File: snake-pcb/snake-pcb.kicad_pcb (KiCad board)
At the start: 4 copper layers, 38.1 x 57.2 mm, 26 parts, among them J1 USB_C, SW1 SW_Push, U1 STM32F072CBT6, U3 XC6206, U4 USBLC6-2SC6

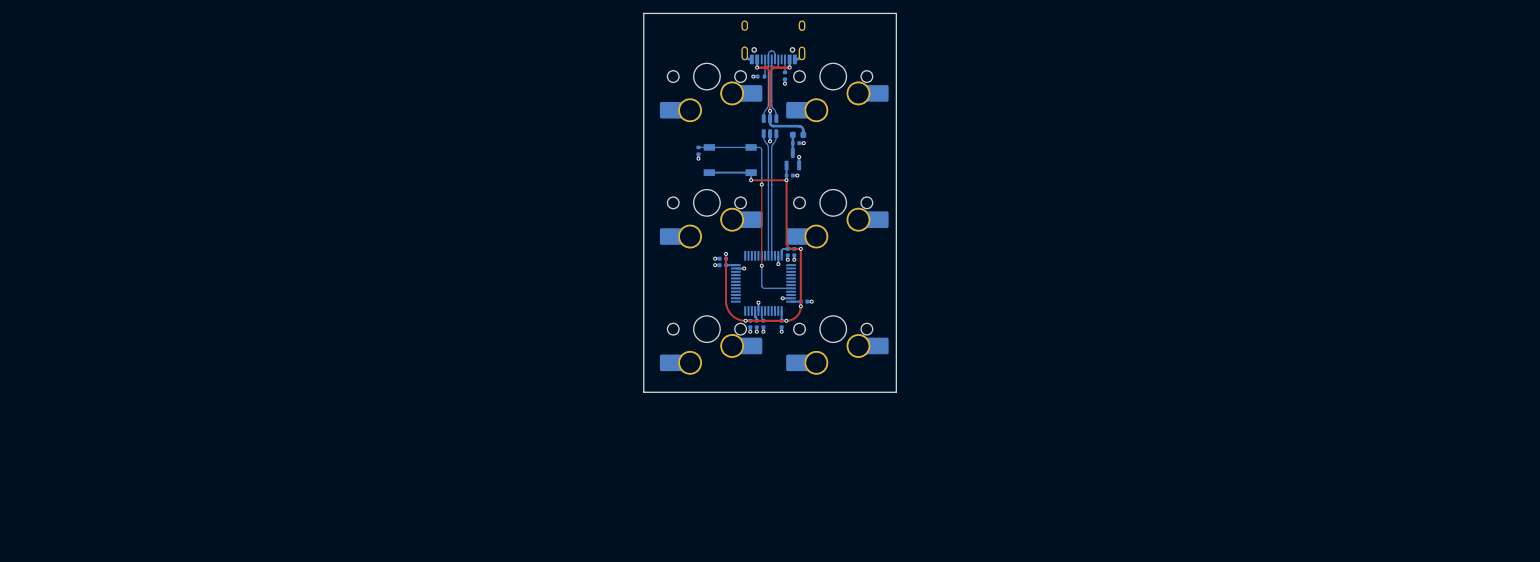
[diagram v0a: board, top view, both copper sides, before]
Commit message: pcb almost finished!
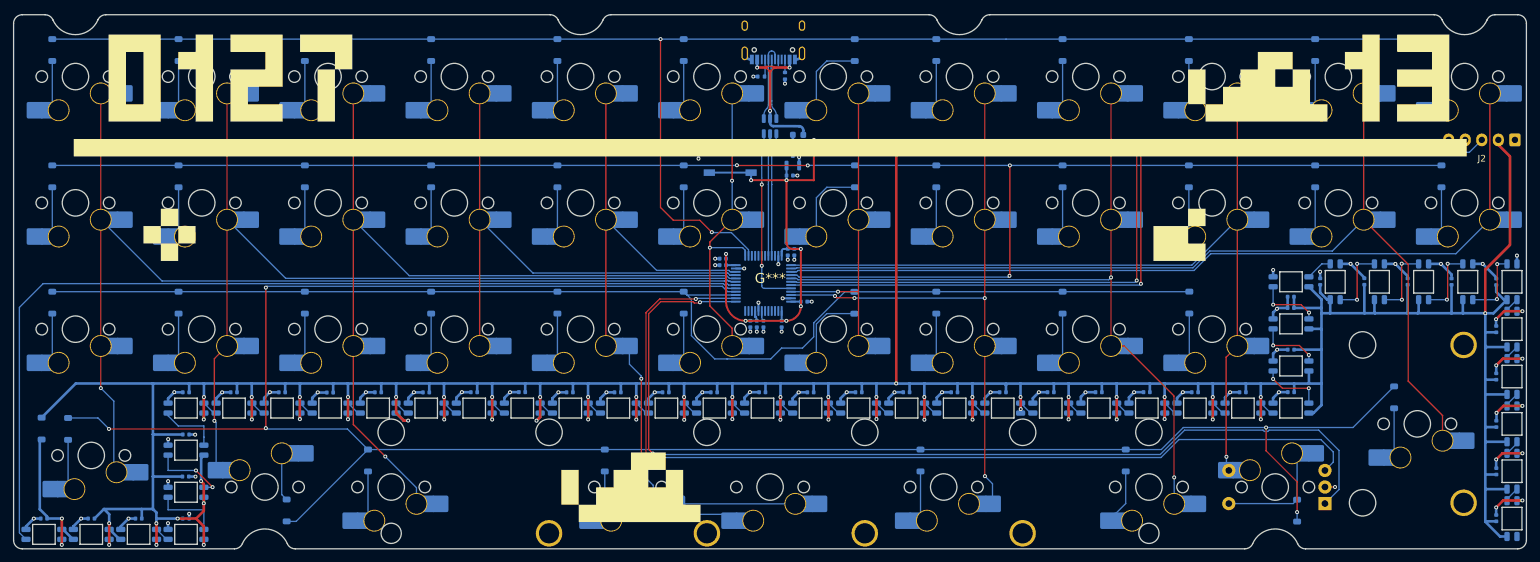
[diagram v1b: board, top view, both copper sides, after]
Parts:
- removed REF** (x6): MX_1.00u_PG151101S11, ScottoKeebs_Scotto:MX_Hotswap_1.00u
- added CapLED1: 100nF, ScottoKeebs_Components:Capacitor_0402, B.Cu at (41.6, 146.6)
- added CapLED10: 100nF, ScottoKeebs_Components:Capacitor_0402, B.Cu at (84.8, 127.6)
- added CapLED11: 100nF, ScottoKeebs_Components:Capacitor_0402, B.Cu at (92.0, 127.6)
- added CapLED12: 100nF, ScottoKeebs_Components:Capacitor_0402, B.Cu at (99.3, 127.6)
- added CapLED13: 100nF, ScottoKeebs_Components:Capacitor_0402, B.Cu at (106.5, 127.6)
- added CapLED14: 100nF, ScottoKeebs_Components:Capacitor_0402, B.Cu at (113.7, 127.5)
- added CapLED15: 100nF, ScottoKeebs_Components:Capacitor_0402, B.Cu at (120.9, 127.6)
- added CapLED16: 100nF, ScottoKeebs_Components:Capacitor_0402, B.Cu at (128.2, 127.6)
- added CapLED17: 100nF, ScottoKeebs_Components:Capacitor_0402, B.Cu at (135.4, 127.6)
- added CapLED18: 100nF, ScottoKeebs_Components:Capacitor_0402, B.Cu at (142.7, 127.6)
- added CapLED19: 100nF, ScottoKeebs_Components:Capacitor_0402, B.Cu at (150.0, 127.6)
- added CapLED2: 100nF, ScottoKeebs_Components:Capacitor_0402, B.Cu at (48.8, 146.6)
- added CapLED20: 100nF, ScottoKeebs_Components:Capacitor_0402, B.Cu at (157.3, 127.6)
- added CapLED21: 100nF, ScottoKeebs_Components:Capacitor_0402, B.Cu at (164.5, 127.6)
- added CapLED22: 100nF, ScottoKeebs_Components:Capacitor_0402, B.Cu at (171.7, 127.6)
- added CapLED23: 100nF, ScottoKeebs_Components:Capacitor_0402, B.Cu at (179.0, 127.6)
- added CapLED24: 100nF, ScottoKeebs_Components:Capacitor_0402, B.Cu at (186.3, 127.6)
- added CapLED25: 100nF, ScottoKeebs_Components:Capacitor_0402, B.Cu at (193.5, 127.6)
- added CapLED26: 100nF, ScottoKeebs_Components:Capacitor_0402, B.Cu at (200.7, 127.6)
- added CapLED27: 100nF, ScottoKeebs_Components:Capacitor_0402, B.Cu at (208.0, 127.6)
- added CapLED28: 100nF, ScottoKeebs_Components:Capacitor_0402, B.Cu at (215.3, 127.6)
- added CapLED29: 100nF, ScottoKeebs_Components:Capacitor_0402, B.Cu at (222.5, 127.6)
- added CapLED3: 100nF, ScottoKeebs_Components:Capacitor_0402, B.Cu at (55.9, 146.6)
- added CapLED30: 100nF, ScottoKeebs_Components:Capacitor_0402, B.Cu at (229.7, 127.6)
- added CapLED31: 100nF, ScottoKeebs_Components:Capacitor_0402, B.Cu at (229.7, 121.1)
- added CapLED32: 100nF, ScottoKeebs_Components:Capacitor_0402, B.Cu at (229.7, 114.9)
- added CapLED33: 100nF, ScottoKeebs_Components:Capacitor_0402, B.Cu at (229.7, 113.2)
- added CapLED34: 100nF, ScottoKeebs_Components:Capacitor_0402, B.Cu at (234.1, 110.9)
- added CapLED35: 100nF, ScottoKeebs_Components:Capacitor_0402, B.Cu at (240.8, 110.9)
- added CapLED36: 100nF, ScottoKeebs_Components:Capacitor_0402, B.Cu at (247.3, 110.9)
- added CapLED37: 100nF, ScottoKeebs_Components:Capacitor_0402, B.Cu at (254.0, 110.9)
- added CapLED38: 100nF, ScottoKeebs_Components:Capacitor_0402, B.Cu at (260.7, 110.9)
- added CapLED39: 100nF, ScottoKeebs_Components:Capacitor_0402, B.Cu at (260.7, 118.1)
- added CapLED4: 100nF, ScottoKeebs_Components:Capacitor_0402, B.Cu at (63.1, 146.6)
- added CapLED40: 100nF, ScottoKeebs_Components:Capacitor_0402, B.Cu at (260.7, 125.2)
- added CapLED41: 100nF, ScottoKeebs_Components:Capacitor_0402, B.Cu at (260.7, 132.3)
- added CapLED42: 100nF, ScottoKeebs_Components:Capacitor_0402, B.Cu at (260.7, 139.5)
- added CapLED43: 100nF, ScottoKeebs_Components:Capacitor_0402, B.Cu at (260.7, 146.6)
- added CapLED5: 100nF, ScottoKeebs_Components:Capacitor_0402, B.Cu at (63.0, 140.3)
- added CapLED6: 100nF, ScottoKeebs_Components:Capacitor_0402, B.Cu at (63.1, 133.9)
- added CapLED7: 100nF, ScottoKeebs_Components:Capacitor_0402, B.Cu at (63.1, 127.6)
- added CapLED8: 100nF, ScottoKeebs_Components:Capacitor_0402, B.Cu at (70.3, 127.6)
- added CapLED9: 100nF, ScottoKeebs_Components:Capacitor_0402, B.Cu at (77.5, 127.6)
- added D1: 1N4148W, Diode_SMD:D_SOD-123, B.Cu at (42.9, 76.0)
- added D10: 1N4148W, Diode_SMD:D_SOD-123, B.Cu at (214.3, 76.0)
- added D11: 1N4148W, Diode_SMD:D_SOD-123, B.Cu at (233.4, 76.0)
- added D12: 1N4148W, Diode_SMD:D_SOD-123, B.Cu at (252.4, 76.0)
- added D13: 1N4148W, Diode_SMD:D_SOD-123, B.Cu at (42.9, 95.0)
- added D14: 1N4148W, Diode_SMD:D_SOD-123, B.Cu at (61.9, 95.0)
- added D15: 1N4148W, Diode_SMD:D_SOD-123, B.Cu at (81.0, 95.0)
- added D16: 1N4148W, Diode_SMD:D_SOD-123, B.Cu at (100.0, 95.0)
- added D17: 1N4148W, Diode_SMD:D_SOD-123, B.Cu at (119.1, 95.0)
- added D18: 1N4148W, Diode_SMD:D_SOD-123, B.Cu at (138.1, 95.0)
- added D19: 1N4148W, Diode_SMD:D_SOD-123, B.Cu at (164.0, 95.0)
- added D2: 1N4148W, Diode_SMD:D_SOD-123, B.Cu at (61.9, 76.0)
- added D20: 1N4148W, Diode_SMD:D_SOD-123, B.Cu at (176.2, 95.0)
- added D21: 1N4148W, Diode_SMD:D_SOD-123, B.Cu at (195.3, 95.0)
- added D22: 1N4148W, Diode_SMD:D_SOD-123, B.Cu at (214.3, 95.0)
- added D23: 1N4148W, Diode_SMD:D_SOD-123, B.Cu at (233.4, 95.0)
- added D24: 1N4148W, Diode_SMD:D_SOD-123, B.Cu at (252.4, 95.0)
- added D25: 1N4148W, Diode_SMD:D_SOD-123, B.Cu at (42.9, 114.1)
- added D26: 1N4148W, Diode_SMD:D_SOD-123, B.Cu at (61.9, 114.1)
- added D27: 1N4148W, Diode_SMD:D_SOD-123, B.Cu at (81.0, 114.1)
- added D28: 1N4148W, Diode_SMD:D_SOD-123, B.Cu at (100.0, 114.1)
- added D29: 1N4148W, Diode_SMD:D_SOD-123, B.Cu at (119.1, 114.1)
- added D3: 1N4148W, Diode_SMD:D_SOD-123, B.Cu at (81.0, 76.0)
- added D30: 1N4148W, Diode_SMD:D_SOD-123, B.Cu at (138.1, 114.1)
- added D31: 1N4148W, Diode_SMD:D_SOD-123, B.Cu at (163.9, 114.1)
- added D32: 1N4148W, Diode_SMD:D_SOD-123, B.Cu at (176.2, 114.1)
- added D33: 1N4148W, Diode_SMD:D_SOD-123, B.Cu at (195.3, 114.1)
- added D34: 1N4148W, Diode_SMD:D_SOD-123, B.Cu at (214.4, 114.0)
- added D35: 1N4148W, Diode_SMD:D_SOD-123, B.Cu at (245.3, 128.3)
- added D36: 1N4148W, Diode_SMD:D_SOD-123, B.Cu at (45.3, 133.1)
- added D37: 1N4148W, Diode_SMD:D_SOD-123, B.Cu at (78.2, 145.4)
- added D38: 1N4148W, Diode_SMD:D_SOD-123, B.Cu at (90.5, 137.9)
- added D39: 1N4148W, Diode_SMD:D_SOD-123, B.Cu at (126.2, 137.9)
- added D4: 1N4148W, Diode_SMD:D_SOD-123, B.Cu at (100.0, 76.0)
- added D40: 1N4148W, Diode_SMD:D_SOD-123, B.Cu at (173.9, 137.9)
- added D41: 1N4148W, Diode_SMD:D_SOD-123, B.Cu at (204.8, 137.9)
- added D42: 1N4148W, Diode_SMD:D_SOD-123, B.Cu at (230.7, 145.4)
- added D5: 1N4148W, Diode_SMD:D_SOD-123, B.Cu at (119.1, 76.0)
- added D6: 1N4148W, Diode_SMD:D_SOD-123, B.Cu at (138.1, 76.0)
- added D7: 1N4148W, Diode_SMD:D_SOD-123, B.Cu at (163.9, 76.0)
- added D8: 1N4148W, Diode_SMD:D_SOD-123, B.Cu at (176.2, 76.0)
- added D9: 1N4148W, Diode_SMD:D_SOD-123, B.Cu at (195.3, 76.0)
- added DLED1: 1N4148W, Diode_SMD:D_SOD-123, B.Cu at (41.3, 133.0)
- added G***: LOGO, snake:snake, F.Cu at (151.2, 110.4)
- added J2: Conn_01x05_Socket, Connector_JST:JST_EH_B5B-EH-A_1x05_P2.50mm_Vertical, F.Cu at (263.5, 89.5)
- added LED1: SK6812MINI, ScottoKeebs_Components:LED_SK6812MINI, B.Cu at (41.6, 149.0)
- added LED10: SK6812MINI, ScottoKeebs_Components:LED_SK6812MINI, B.Cu at (84.8, 130.0)
- added LED11: SK6812MINI, ScottoKeebs_Components:LED_SK6812MINI, B.Cu at (92.0, 130.0)
- added LED12: SK6812MINI, ScottoKeebs_Components:LED_SK6812MINI, B.Cu at (99.3, 130.0)
- added LED13: SK6812MINI, ScottoKeebs_Components:LED_SK6812MINI, B.Cu at (106.5, 130.0)
- added LED14: SK6812MINI, ScottoKeebs_Components:LED_SK6812MINI, B.Cu at (113.8, 130.0)
- added LED15: SK6812MINI, ScottoKeebs_Components:LED_SK6812MINI, B.Cu at (121.0, 130.0)
- added LED16: SK6812MINI, ScottoKeebs_Components:LED_SK6812MINI, B.Cu at (128.3, 130.0)
- added LED17: SK6812MINI, ScottoKeebs_Components:LED_SK6812MINI, B.Cu at (135.5, 130.0)
- added LED18: SK6812MINI, ScottoKeebs_Components:LED_SK6812MINI, B.Cu at (142.8, 130.0)
- added LED19: SK6812MINI, ScottoKeebs_Components:LED_SK6812MINI, B.Cu at (150.0, 130.0)
- added LED2: SK6812MINI, ScottoKeebs_Components:LED_SK6812MINI, B.Cu at (48.8, 149.0)
- added LED20: SK6812MINI, ScottoKeebs_Components:LED_SK6812MINI, B.Cu at (157.3, 130.0)
- added LED21: SK6812MINI, ScottoKeebs_Components:LED_SK6812MINI, B.Cu at (164.5, 130.0)
- added LED22: SK6812MINI, ScottoKeebs_Components:LED_SK6812MINI, B.Cu at (171.8, 130.0)
- added LED23: SK6812MINI, ScottoKeebs_Components:LED_SK6812MINI, B.Cu at (179.0, 130.0)
- added LED24: SK6812MINI, ScottoKeebs_Components:LED_SK6812MINI, B.Cu at (186.3, 130.0)
- added LED25: SK6812MINI, ScottoKeebs_Components:LED_SK6812MINI, B.Cu at (193.5, 130.0)
- added LED26: SK6812MINI, ScottoKeebs_Components:LED_SK6812MINI, B.Cu at (200.7, 130.0)
- added LED27: SK6812MINI, ScottoKeebs_Components:LED_SK6812MINI, B.Cu at (208.0, 130.0)
- added LED28: SK6812MINI, ScottoKeebs_Components:LED_SK6812MINI, B.Cu at (215.2, 130.0)
- added LED29: SK6812MINI, ScottoKeebs_Components:LED_SK6812MINI, B.Cu at (222.5, 130.0)
- added LED3: SK6812MINI, ScottoKeebs_Components:LED_SK6812MINI, B.Cu at (55.9, 149.0)
- added LED30: SK6812MINI, ScottoKeebs_Components:LED_SK6812MINI, B.Cu at (229.7, 130.0)
- added LED31: SK6812MINI, ScottoKeebs_Components:LED_SK6812MINI, B.Cu at (229.7, 123.6)
- added LED32: SK6812MINI, ScottoKeebs_Components:LED_SK6812MINI, B.Cu at (229.7, 117.3)
- added LED33: SK6812MINI, ScottoKeebs_Components:LED_SK6812MINI, B.Cu at (229.7, 110.9)
- added LED34: SK6812MINI, ScottoKeebs_Components:LED_SK6812MINI, B.Cu at (236.4, 110.9)
- added LED35: SK6812MINI, ScottoKeebs_Components:LED_SK6812MINI, B.Cu at (243.1, 110.9)
- added LED36: SK6812MINI, ScottoKeebs_Components:LED_SK6812MINI, B.Cu at (249.7, 110.9)
- added LED37: SK6812MINI, ScottoKeebs_Components:LED_SK6812MINI, B.Cu at (256.4, 110.9)
- added LED38: SK6812MINI, ScottoKeebs_Components:LED_SK6812MINI, B.Cu at (263.1, 110.9)
- added LED39: SK6812MINI, ScottoKeebs_Components:LED_SK6812MINI, B.Cu at (263.1, 118.1)
- added LED4: SK6812MINI, ScottoKeebs_Components:LED_SK6812MINI, B.Cu at (63.1, 149.0)
- added LED40: SK6812MINI, ScottoKeebs_Components:LED_SK6812MINI, B.Cu at (263.1, 125.2)
- added LED41: SK6812MINI, ScottoKeebs_Components:LED_SK6812MINI, B.Cu at (263.1, 132.3)
- added LED42: SK6812MINI, ScottoKeebs_Components:LED_SK6812MINI, B.Cu at (263.1, 139.5)
- added LED43: SK6812MINI, ScottoKeebs_Components:LED_SK6812MINI, B.Cu at (263.1, 146.6)
- added LED5: SK6812MINI, ScottoKeebs_Components:LED_SK6812MINI, B.Cu at (63.1, 142.7)
- added LED6: SK6812MINI, ScottoKeebs_Components:LED_SK6812MINI, B.Cu at (63.1, 136.3)
- added LED7: SK6812MINI, ScottoKeebs_Components:LED_SK6812MINI, B.Cu at (63.1, 130.0)
- added LED8: SK6812MINI, ScottoKeebs_Components:LED_SK6812MINI, B.Cu at (70.3, 130.0)
- added LED9: SK6812MINI, ScottoKeebs_Components:LED_SK6812MINI, B.Cu at (77.6, 130.0)
- added MX1: MX_SW_solder, PCM_marbastlib-mx:SW_MX_HS_CPG151101S11_1u, B.Cu at (46.4, 80.0)
- added MX10: MX_SW_solder, PCM_marbastlib-mx:SW_MX_HS_CPG151101S11_1u, B.Cu at (217.8, 80.0)
- added MX11: MX_SW_solder, PCM_marbastlib-mx:SW_MX_HS_CPG151101S11_1u, B.Cu at (236.9, 80.0)
- added MX12: MX_SW_solder, PCM_marbastlib-mx:SW_MX_HS_CPG151101S11_1u, B.Cu at (255.9, 80.0)
- added MX13: MX_SW_solder, PCM_marbastlib-mx:SW_MX_HS_CPG151101S11_1u, B.Cu at (46.4, 99.0)
- added MX14: MX_SW_solder, PCM_marbastlib-mx:SW_MX_HS_CPG151101S11_1u, B.Cu at (65.4, 99.0)
- added MX15: MX_SW_solder, PCM_marbastlib-mx:SW_MX_HS_CPG151101S11_1u, B.Cu at (84.5, 99.0)
- added MX16: MX_SW_solder, PCM_marbastlib-mx:SW_MX_HS_CPG151101S11_1u, B.Cu at (103.5, 99.0)
- added MX17: MX_SW_solder, PCM_marbastlib-mx:SW_MX_HS_CPG151101S11_1u, B.Cu at (122.6, 99.0)
- added MX18: MX_SW_solder, PCM_marbastlib-mx:SW_MX_HS_CPG151101S11_1u, B.Cu at (141.6, 99.0)
- added MX19: MX_SW_solder, PCM_marbastlib-mx:SW_MX_HS_CPG151101S11_1u, B.Cu at (160.7, 99.0)
- added MX2: MX_SW_solder, PCM_marbastlib-mx:SW_MX_HS_CPG151101S11_1u, B.Cu at (65.4, 80.0)
- added MX20: MX_SW_solder, PCM_marbastlib-mx:SW_MX_HS_CPG151101S11_1u, B.Cu at (179.7, 99.0)
- added MX21: MX_SW_solder, PCM_marbastlib-mx:SW_MX_HS_CPG151101S11_1u, B.Cu at (198.8, 99.0)
- added MX22: MX_SW_solder, PCM_marbastlib-mx:SW_MX_HS_CPG151101S11_1u, B.Cu at (217.8, 99.0)
- added MX23: MX_SW_solder, PCM_marbastlib-mx:SW_MX_HS_CPG151101S11_1u, B.Cu at (236.9, 99.0)
- added MX24: MX_SW_solder, PCM_marbastlib-mx:SW_MX_HS_CPG151101S11_1u, B.Cu at (255.9, 99.0)
- added MX25: MX_SW_solder, PCM_marbastlib-mx:SW_MX_HS_CPG151101S11_1u, B.Cu at (46.4, 118.1)
- added MX26: MX_SW_solder, PCM_marbastlib-mx:SW_MX_HS_CPG151101S11_1u, B.Cu at (65.4, 118.1)
- added MX27: MX_SW_solder, PCM_marbastlib-mx:SW_MX_HS_CPG151101S11_1u, B.Cu at (84.5, 118.1)
- added MX28: MX_SW_solder, PCM_marbastlib-mx:SW_MX_HS_CPG151101S11_1u, B.Cu at (103.5, 118.1)
- added MX29: MX_SW_solder, PCM_marbastlib-mx:SW_MX_HS_CPG151101S11_1u, B.Cu at (122.6, 118.1)
- added MX3: MX_SW_solder, PCM_marbastlib-mx:SW_MX_HS_CPG151101S11_1u, B.Cu at (84.5, 80.0)
- added MX30: MX_SW_solder, PCM_marbastlib-mx:SW_MX_HS_CPG151101S11_1u, B.Cu at (141.6, 118.1)
- added MX31: MX_SW_solder, PCM_marbastlib-mx:SW_MX_HS_CPG151101S11_1u, B.Cu at (160.7, 118.1)
- added MX32: MX_SW_solder, PCM_marbastlib-mx:SW_MX_HS_CPG151101S11_1u, B.Cu at (179.7, 118.1)
- added MX33: MX_SW_solder, PCM_marbastlib-mx:SW_MX_HS_CPG151101S11_1u, B.Cu at (198.8, 118.1)
- added MX34: MX_SW_solder, PCM_marbastlib-mx:SW_MX_HS_CPG151101S11_1u, B.Cu at (217.8, 118.1)
- added MX35: MX_SW_solder, PCM_marbastlib-mx:SW_MX_HS_CPG151101S11_1u, B.Cu at (248.8, 132.3)
- added MX36: MX_SW_solder, PCM_marbastlib-mx:SW_MX_HS_CPG151101S11_1.25u, B.Cu at (48.8, 137.1)
- added MX37: MX_SW_solder, PCM_marbastlib-mx:SW_MX_HS_CPG151101S11_1u, B.Cu at (75.0, 141.9)
- added MX38: MX_SW_solder, PCM_marbastlib-mx:SW_MX_HS_CPG151101S11_1u, B.Cu at (94.0, 141.9)
- added MX39: MX_SW_solder, PCM_marbastlib-mx:SW_MX_HS_CPG151101S11_1u, B.Cu at (129.7, 141.9)
- added MX4: MX_SW_solder, PCM_marbastlib-mx:SW_MX_HS_CPG151101S11_1u, B.Cu at (103.5, 80.0)
- added MX40: MX_SW_solder, PCM_marbastlib-mx:SW_MX_HS_CPG151101S11_1u, B.Cu at (177.4, 141.9)
- added MX41: MX_SW_solder, PCM_marbastlib-mx:SW_MX_HS_CPG151101S11_1u, B.Cu at (208.3, 141.9)
- added MX42: MX_SW_solder, PCM_marbastlib-mx:SW_MX_HS_CPG151101S11_1u, B.Cu at (227.4, 141.9)
- added MX43: MX_SW_solder, PCM_marbastlib-mx:SW_MX_HS_CPG151101S11_1u, B.Cu at (151.2, 141.9)
- added MX5: MX_SW_solder, PCM_marbastlib-mx:SW_MX_HS_CPG151101S11_1u, B.Cu at (122.6, 80.0)
- added MX6: MX_SW_solder, PCM_marbastlib-mx:SW_MX_HS_CPG151101S11_1u, B.Cu at (141.6, 80.0)
- added MX7: MX_SW_solder, PCM_marbastlib-mx:SW_MX_HS_CPG151101S11_1u, B.Cu at (160.7, 80.0)
- added MX8: MX_SW_solder, PCM_marbastlib-mx:SW_MX_HS_CPG151101S11_1u, B.Cu at (179.7, 80.0)
- added MX9: MX_SW_solder, PCM_marbastlib-mx:SW_MX_HS_CPG151101S11_1u, B.Cu at (198.8, 80.0)
- added S35: MX_stab, PCM_marbastlib-mx:STAB_MX_P_ISO-ROT, F.Cu at (248.8, 132.3)
- added S39: MX_stab, PCM_marbastlib-mx:STAB_MX_P_2.75u, F.Cu at (129.7, 141.9)
- added S40: MX_stab, PCM_marbastlib-mx:STAB_MX_P_2.25u, F.Cu at (177.4, 141.9)
- added S43: MX_stab, PCM_marbastlib-mx:STAB_MX_7u, F.Cu at (151.2, 141.9)
- added SW2: RotaryEncoder_Switch, ScottoKeebs_Scotto:Encoder_EC11_MX, F.Cu at (227.4, 141.9)
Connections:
- U1 pad 13: /A3 -> rotA
- U1 pad 14: /A4 -> rotB
- U1 pad 15: /A5 -> row2
- U1 pad 16: /A6 -> row3
- U1 pad 17: /A7 -> data 3.3v
- U1 pad 18: /B0 -> col0
- U1 pad 19: /B1 -> col1
- U1 pad 20: /B2 -> col2
- U1 pad 21: /B10 -> col3
- U1 pad 22: /B11 -> col4
- U1 pad 25: /B12 -> col5
- U1 pad 26: /B13 -> row0
- U1 pad 37: /A14 -> col9
- U1 pad 38: /A15 -> col10
- U1 pad 39: /B3 -> col11
- U1 pad 40: /B4 -> row1
- U1 pad 41: /B5 -> col8
- U1 pad 42: /B6 -> scl
- U1 pad 43: /B7 -> sda
- U1 pad 45: /B8 -> col6
- U1 pad 46: /B9 -> col7
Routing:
- net +5V: track 2.76 -> 681.1 mm, vias 0 -> 57
- net row3: track 0.00 -> 331.5 mm, vias 0 -> 5
- net row1: track 0.00 -> 259.4 mm, vias 0 -> 4
- net row0: track 0.00 -> 251.8 mm, vias 0 -> 2
- net row2: track 0.00 -> 192.5 mm
- net GND: track 20.1 -> 178.9 mm, vias 20 -> 73
- net col0: track 0.00 -> 158.0 mm, vias 0 -> 1
- net rotA: track 0.00 -> 150.8 mm, vias 0 -> 2
- net col10: track 0.00 -> 146.7 mm
- net data 3.3v: track 0.00 -> 145.3 mm
- net rotB: track 0.00 -> 144.8 mm, vias 0 -> 2
- net col1: track 0.00 -> 138.4 mm, vias 0 -> 1
- net col11: track 0.00 -> 127.7 mm
- net col9: track 0.00 -> 127.7 mm, vias 0 -> 1
- net col2: track 0.00 -> 127.2 mm, vias 0 -> 1
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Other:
- board size 38.1 x 57.2 mm -> 228.2 x 80.6 mm
